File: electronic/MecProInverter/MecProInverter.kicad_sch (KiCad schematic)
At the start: 3 parts, among them U1 USB-TYPE-C-007, U2 ESP32-S3-MINI-1-N8, U3 IKCM20L60GA

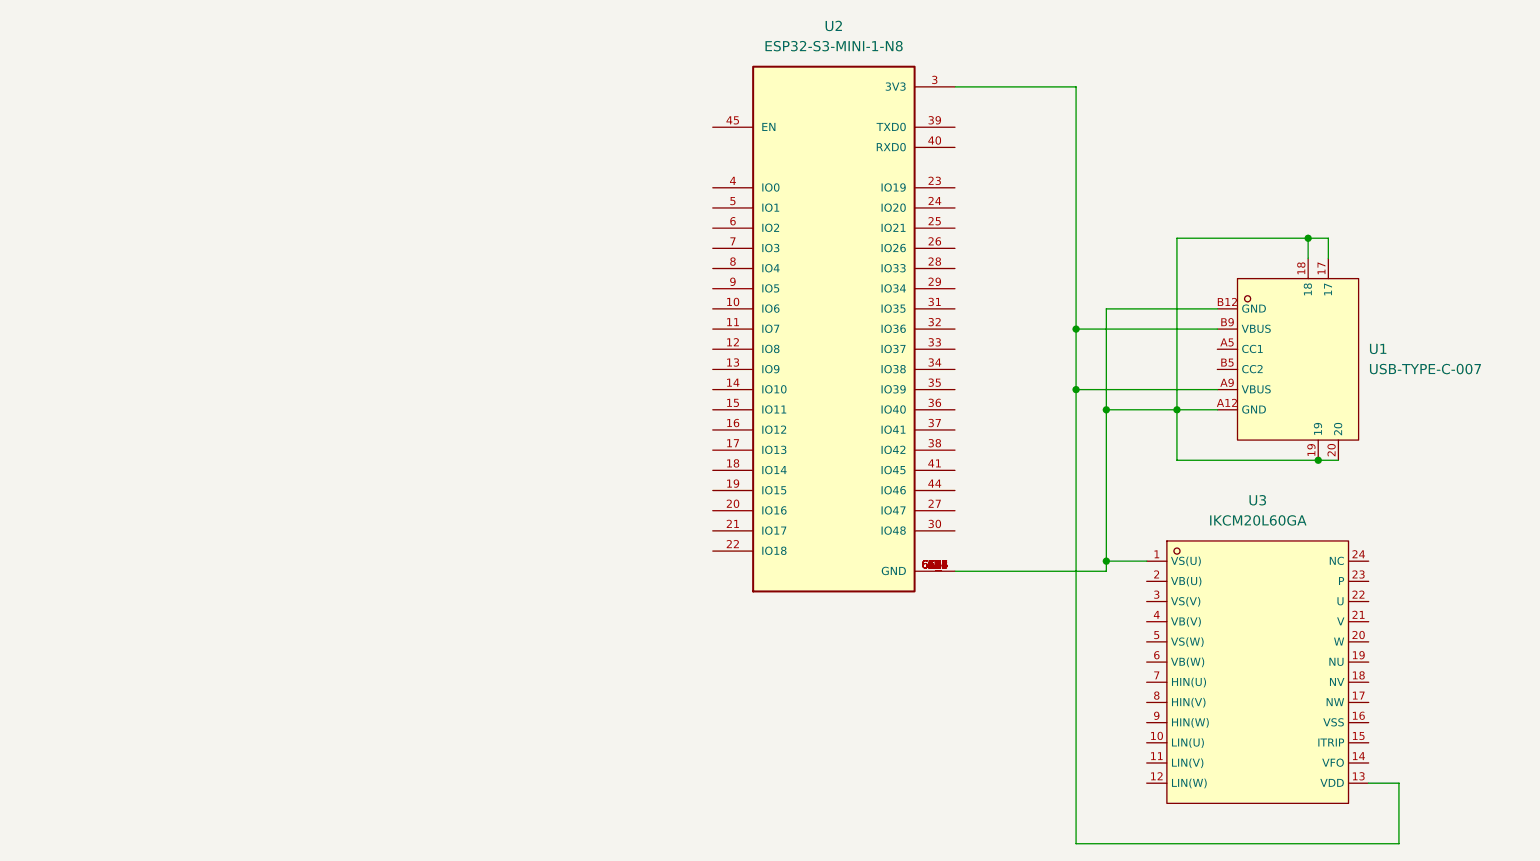
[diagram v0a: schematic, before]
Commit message: electronic
Test .gitignore (venv)
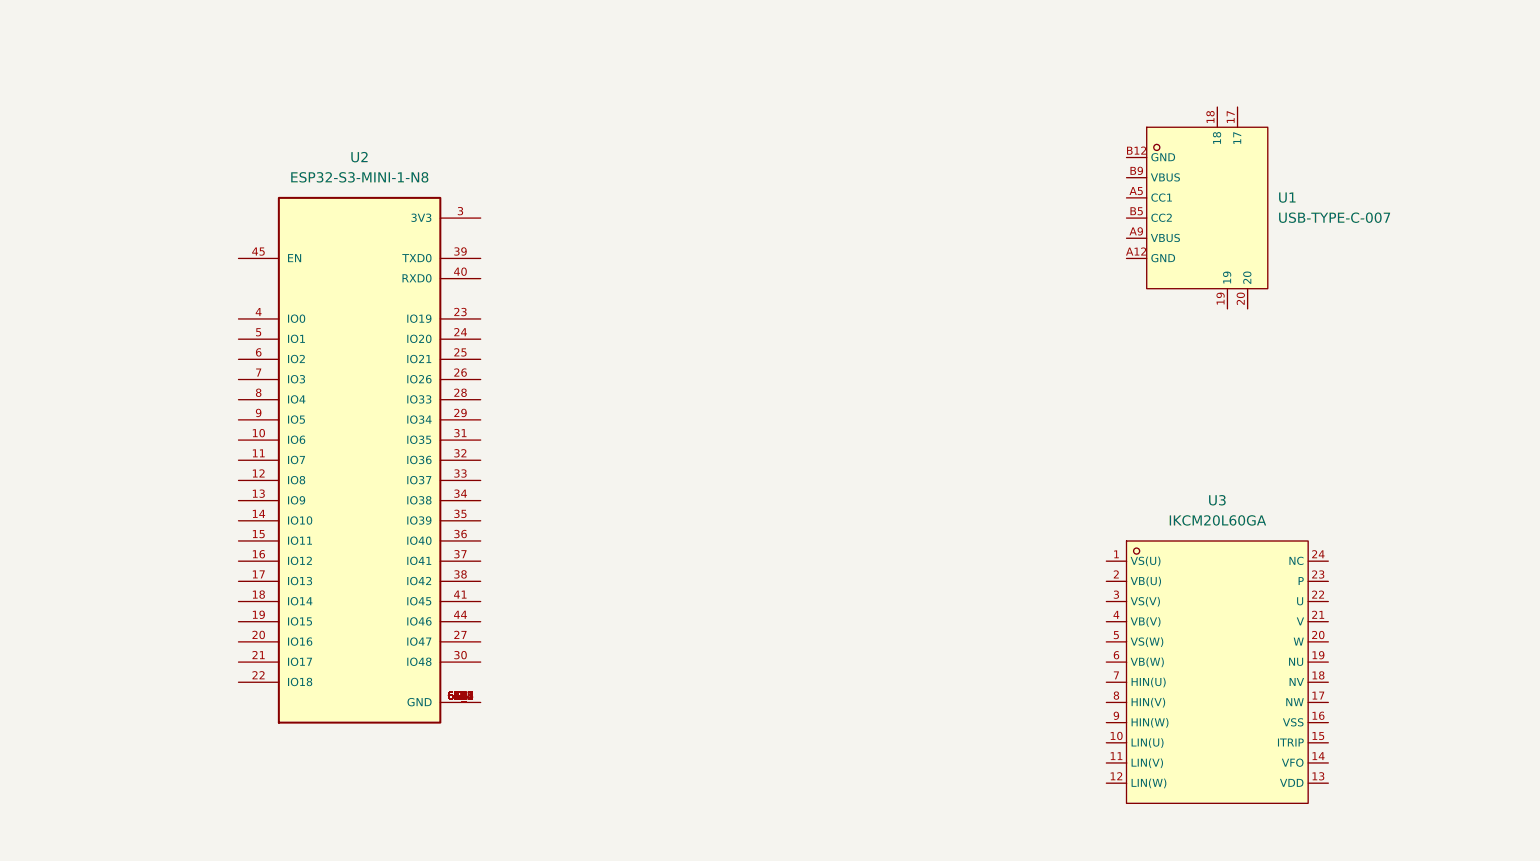
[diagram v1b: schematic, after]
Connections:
- net at U2.1 (GND), U2.2 (GND), U2.42 (GND)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: no longer U1.17, U1.18, U1.19, U1.20, U1.A12 (GND), U1.B12 (GND), U3.1 (VS(U))
- now unconnected: U1.A9 (VBUS), U1.B9 (VBUS), U2.3 (3V3), U3.13 (VDD)
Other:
- moved on the sheet: U1, U2, U3

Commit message: electronic
library expanded
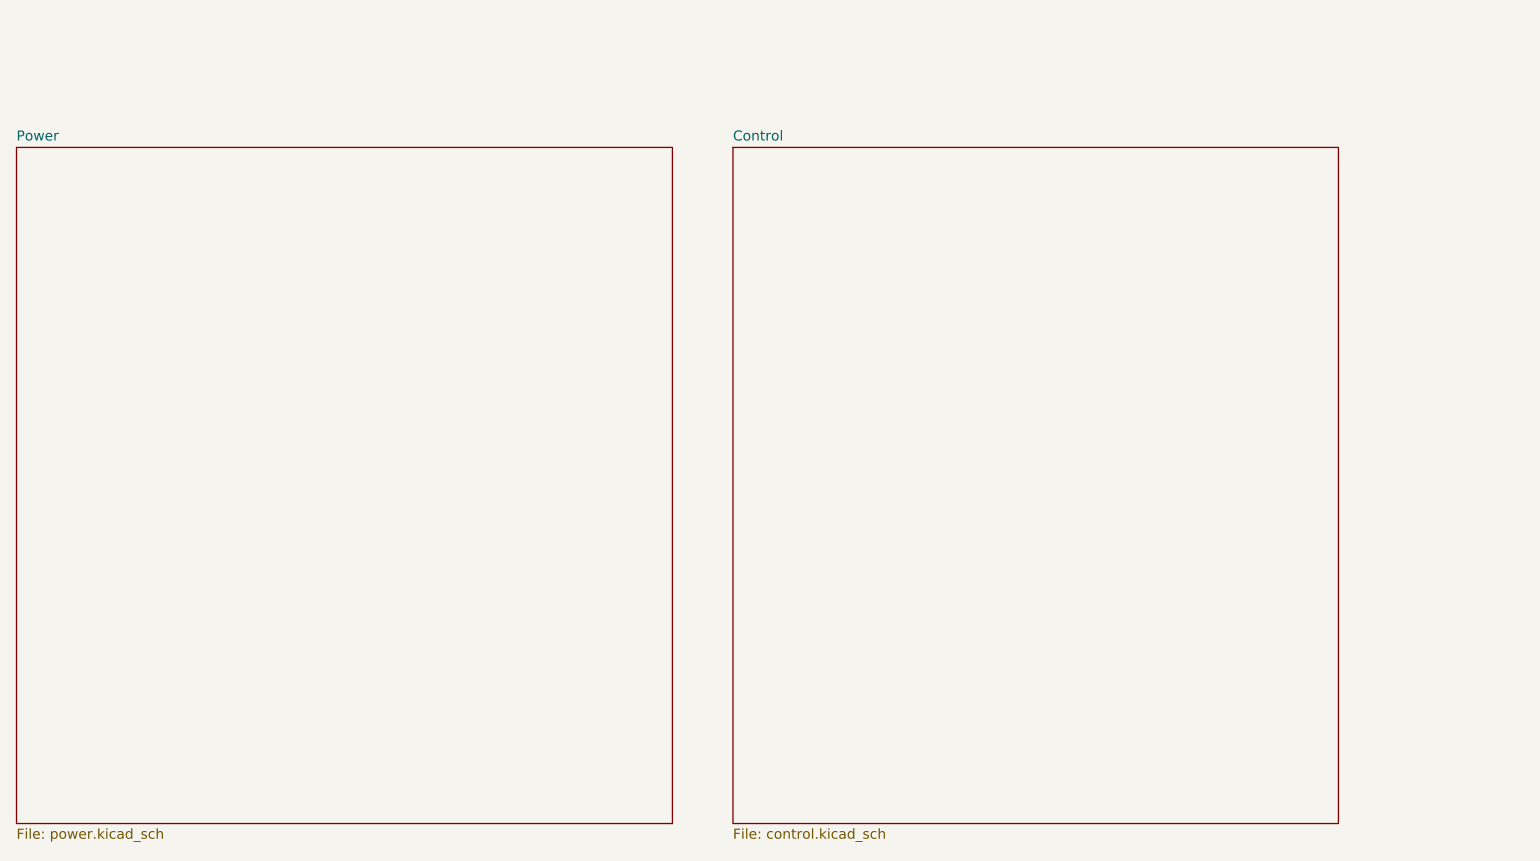
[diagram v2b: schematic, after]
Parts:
- removed U1: USB-TYPE-C-007, footprint:TYPE-C-SMD_USB-TYPE-C-007, symbol USB-TYPE-C-007:USB-TYPE-C-007
- removed U2: ESP32-S3-MINI-1-N8, footprint:BULETM-SMD_ESP32-S3-MINI-1-N8, symbol ESP32-S3-MINI-1-N8:ESP32-S3-MINI-1-N8
- removed U3: IKCM20L60GA, footprint:DIP-24_L36.0-W21.0-P1.60-LS28.6-TL, symbol IKCM20L60GA:IKCM20L60GA
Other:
- added sheet Control (control.kicad_sch)
- added sheet Power (power.kicad_sch)
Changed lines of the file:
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@@
 (kicad_sch (version 20230121) (generator eeschema)
-  (paper "A4")
-  (symbol (lib_id "IKCM20L60GA:IKCM20L60GA") (at 191.77 97.79 0) (unit 1)
-    (in_bom yes) (on_board yes) (dnp no) (fields_autoplaced)
-    (property "Reference" "U3" (at 190.5 74.93 0)
-      (effects (font (size 1.27 1.27)))
+  (paper "A3")
+  (title_block
+    (date "2023-11-04")
+  )
+  (sheet (at 129.54 30.48) (size 76.2 85.09) (fields_autoplaced)
+    (stroke (width 0.1524) (type solid))
+    (fill (color 255 204 0 1.0000))
+    (property "Sheetname" "Control" (at 129.54 29.7684 0)
+      (effects (font (size 1.27 1.27)) (justify left bottom))
     )
-    (property "Value" "IKCM20L60GA" (at 190.5 77.47 0)
-      (effects (font (size 1.27 1.27)))
+    (property "Sheetfile" "control.kicad_sch" (at 129.54 116.1546 0)
+      (effects (font (size 1.27 1.27)) (justify left top))
     )
-    (property "Footprint" "footprint:DIP-24_L36.0-W21.0-P1.60-LS28.6-TL" (at 191.77 107.95 0)
-      (effects (font (size 1.27 1.27) italic) hide)
-    )
-    (property "Datasheet" "https://item.szlcsc.com/556478.html" (at 189.484 97.663 0)
-      (effects (font (size 1.27 1.27)) (justify left) hide)
-    )
-    (property "LCSC" "C536161" (at 191.77 97.79 0)
-      (effects (font (size 1.27 1.27)) hide)
-    )
-    (pin "1")
-    (pin "10")
-    (pin "11")
-    (pin "12")
-    (pin "13")
-    (pin "14")
-    (pin "15")
-    (pin "16")
-    (pin "17")
-    (pin "18")
-    (pin "19")
-    (pin "2")
-    (pin "20")
-    (pin "21")
-    (pin "22")
-    (pin "23")
-    (pin "24")
-    (pin "3")
-    (pin "4")
-    (pin "5")
-    (pin "6")
-    (pin "7")
-    (pin "8")
-    (pin "9")
     (instances
       (project "MecProInverter"
-        (path "/c9071429-8b0d-45bf-aa6d-71cc2b7f068c"
-          (reference "U3") (unit 1)
-        )
+        (path "/c9071429-8b0d-45bf-aa6d-71cc2b7f068c" (page "3"))
       )
     )
   )
-  (symbol (lib_id "ESP32-S3-MINI-1-N8:ESP32-S3-MINI-1-N8") (at 82.55 69.85 0) (unit 1)
-    (in_bom yes) (on_board yes) (dnp no) (fields_autoplaced)
-    (property "Reference" "U2" (at 82.55 31.75 0)
-      (effects (font (size 1.27 1.27)))
+  (sheet (at 39.37 30.48) (size 82.55 85.09) (fields_autoplaced)
+    (stroke (width 0.1524) (type solid))
+    (fill (color 0 0 255 1.0000))
+    (property "Sheetname" "Power" (at 39.37 29.7684 0)
+      (effects (font (size 1.27 1.27)) (justify left bottom))
     )
-    (property "Value" "ESP32-S3-MINI-1-N8" (at 82.55 34.29 0)
-      (effects (font (size 1.27 1.27)))
+    (property "Sheetfile" "power.kicad_sch" (at 39.37 116.1546 0)
+      (effects (font (size 1.27 1.27)) (justify left top))
     )
-    (property "Footprint" "footprint:BULETM-SMD_ESP32-S3-MINI-1-N8" (at 82.55 69.85 0)
-      (effects (font (size 1.27 1.27)) (justify bottom) hide)
-    )
-    (property "Datasheet" "" (at 82.55 69.85 0)
-      (effects (font (size 1.27 1.27)) hide)
-    )
-    (property "MF" "Espressif Systems" (at 82.55 69.85 0)
-      (effects (font (size 1.27 1.27)) (justify bottom) hide)
-    )
-    (property "MAXIMUM_PACKAGE_HEIGHT" "2.55mm" (at 82.55 69.85 0)
-      (effects (font (size 1.27 1.27)) (justify bottom) hide)
-    )
-    (property "Package" "None" (at 82.55 69.85 0)
-      (effects (font (size 1.27 1.27)) (justify bottom) hide)
-    )
-    (property "Price" "None" (at 82.55 69.85 0)
-      (effects (font (size 1.27 1.27)) (justify bottom) hide)
-    )
-    (property "Check_prices" "https://www.snapeda.com/parts/ESP32-S3-MINI-1-N8/Espressif+Systems/view-part/?ref=eda" (at 82.55 69.85 0)
-      (effects (font (size 1.27 1.27)) (justify bottom) hide)
-    )
-    (property "STANDARD" "Manufacturer Recommendations" (at 82.55 69.85 0)
-      (effects (font (size 1.27 1.27)) (justify bottom) hide)
-    )
-    (property "PARTREV" "v0.6" (at 82.55 69.85 0)
-      (effects (font (size 1.27 1.27)) (justify bottom) hide)
-    )
-    (property "SnapEDA_Link" "https://www.snapeda.com/parts/ESP32-S3-MINI-1-N8/Espressif+Systems/view-part/?ref=snap" (at 82.55 69.85 0)
-      (effects (font (size 1.27 1.27)) (justify bottom) hide)
-    )
-    (property "MP" "ESP32-S3-MINI-1-N8" (at 82.55 69.85 0)
-      (effects (font (size 1.27 1.27)) (justify bottom) hide)
-    )
-    (property "Purchase-URL" "https://www.snapeda.com/api/url_track_click_mouser/?unipart_id=8941370&manufacturer=Espressif Systems&part_name=ESP32-S3-MINI-1-N8&search_term=None" (at 82.55 69.85 0)
-      (effects (font (size 1.27 1.27)) (justify bottom) hide)
-    )
-    (property "Description" "\nBluetooth, WiFi 802.11b/g/n, Bluetooth v5.0 Transceiver Module 2.4GHz PCB Trace Surface Mount\n" (at 82.55 69.85 0)
-      (effects (font (size 1.27 1.27)) (justify bottom) hide)
-    )
-    (property "Availability" "In Stock" (at 82.55 69.85 0)
-      (effects (font (size 1.27 1.27)) (justify bottom) hide)
-    )
-    (property "MANUFACTURER" "Espressif" (at 82.55 69.85 0)
-      (effects (font (size 1.27 1.27)) (justify bottom) hide)
-    )
-    (pin "1")
-    (pin "10")
-    (pin "11")
-    (pin "12")
-    (pin "13")
-    (pin "14")
-    (pin "15")
-    (pin "16")
-    (pin "17")
-    (pin "18")
-    (pin "19")
-    (pin "2")
-    (pin "20")
-    (pin "21")
-    (pin "22")
-    (pin "23")
-    (pin "24")
-    (pin "25")
-    (pin "26")
-    (pin "27")
-    (pin "28")
-    (pin "29")
-    (pin "3")
-    (pin "30")
-    (pin "31")
-    (pin "32")
-    (pin "33")
-    (pin "34")
-    (pin "35")
-    (pin "36")
-    (pin "37")
-    (pin "38")
-    (pin "39")
-    (pin "4")
-    (pin "40")
-    (pin "41")
-    (pin "42")
-    (pin "43")
-    (pin "44")
-    (pin "45")
-    (pin "46")
-    (pin "47")
-    (pin "48")
-    (pin "49")
-    (pin "5")
-    (pin "50")
-    (pin "51")
-    (pin "52")
-    (pin "53")
-    (pin "54")
-    (pin "55")
-    (pin "56")
-    (pin "57")
-    (pin "58")
-    (pin "59")
-    (pin "6")
-    (pin "60")
-    (pin "61")
-    (pin "61_1")
-    (pin "61_2")
-    (pin "61_3")
-    (pin "61_4")
-    (pin "61_5")
-    (pin "61_6")
-    (pin "61_7")
-    (pin "61_8")
-    (pin "62")
-    (pin "63")
-    (pin "64")
-    (pin "65")
-    (pin "7")
-    (pin "8")
-    (pin "9")
     (instances
       (project "MecProInverter"
-        (path "/c9071429-8b0d-45bf-aa6d-71cc2b7f068c"
-          (reference "U2") (unit 1)
-        )
+        (path "/c9071429-8b0d-45bf-aa6d-71cc2b7f068c" (page "2"))
       )
     )
-  )
-  (symbol (lib_id "USB-TYPE-C-007:USB-TYPE-C-007") (at 187.96 38.1 0) (unit 1)
-    (in_bom yes) (on_board yes) (dnp no) (fields_autoplaced)
-    (property "Reference" "U1" (at 198.12 36.83 0)
-      (effects (font (size 1.27 1.27)) (justify left))
-    )
-    (property "Value" "USB-TYPE-C-007" (at 198.12 39.37 0)
-      (effects (font (size 1.27 1.27)) (justify left))
-    )
-    (property "Footprint" "footprint:TYPE-C-SMD_USB-TYPE-C-007" (at 187.96 48.26 0)
-      (effects (font (size 1.27 1.27) italic) hide)
-    )
-    (property "Datasheet" "https://atta.szlcsc.com/upload/public/pdf/source/20211217/F345BBF13C3CEC304DBEB8D87DF0AF9A.pdf" (at 185.674 37.973 0)
-      (effects (font (size 1.27 1.27)) (justify left) hide)
-    )
-    (property "LCSC" "C2927027" (at 187.96 38.1 0)
-      (effects (font (size 1.27 1.27)) hide)
-    )
-    (pin "17")
-    (pin "18")
-    (pin "19")
-    (pin "20")
-    (pin "A12")
-    (pin "A5")
-    (pin "A9")
-    (pin "B12")
-    (pin "B5")
-    (pin "B9")
-    (instances
-      (project "MecProInverter"
-        (path "/c9071429-8b0d-45bf-aa6d-71cc2b7f068c"
-          (reference "U1") (unit 1)
-        )
-      )
-    )
